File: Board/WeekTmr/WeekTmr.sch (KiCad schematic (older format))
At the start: 18 parts, among them J1 Screw_Terminal_01x03, J2 Screw_Terminal_01x03, J3 Barrel_Jack_MountingPin, J4 DS3231, K1 DIPxx-1Cxx-51x, K2 DIPxx-1Cxx-51x, Q1 BC817, Q2 BC817, SW1 DOWN_BUT, SW2 UP_BUT, SW3 SELECT_BUT, U1 NHD-0420H1Z

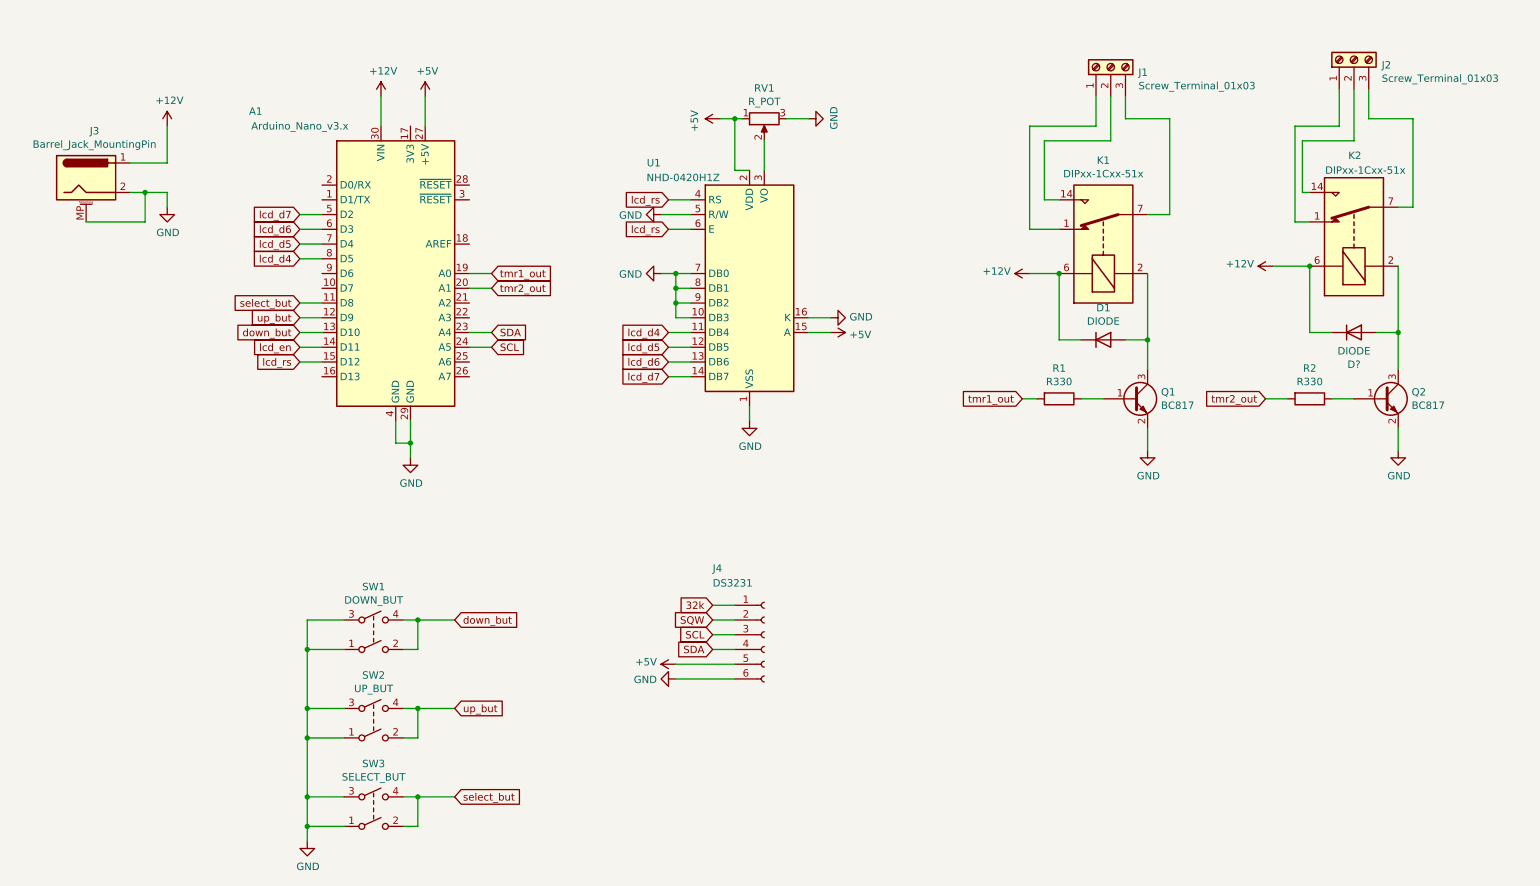
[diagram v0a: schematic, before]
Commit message: pcb update
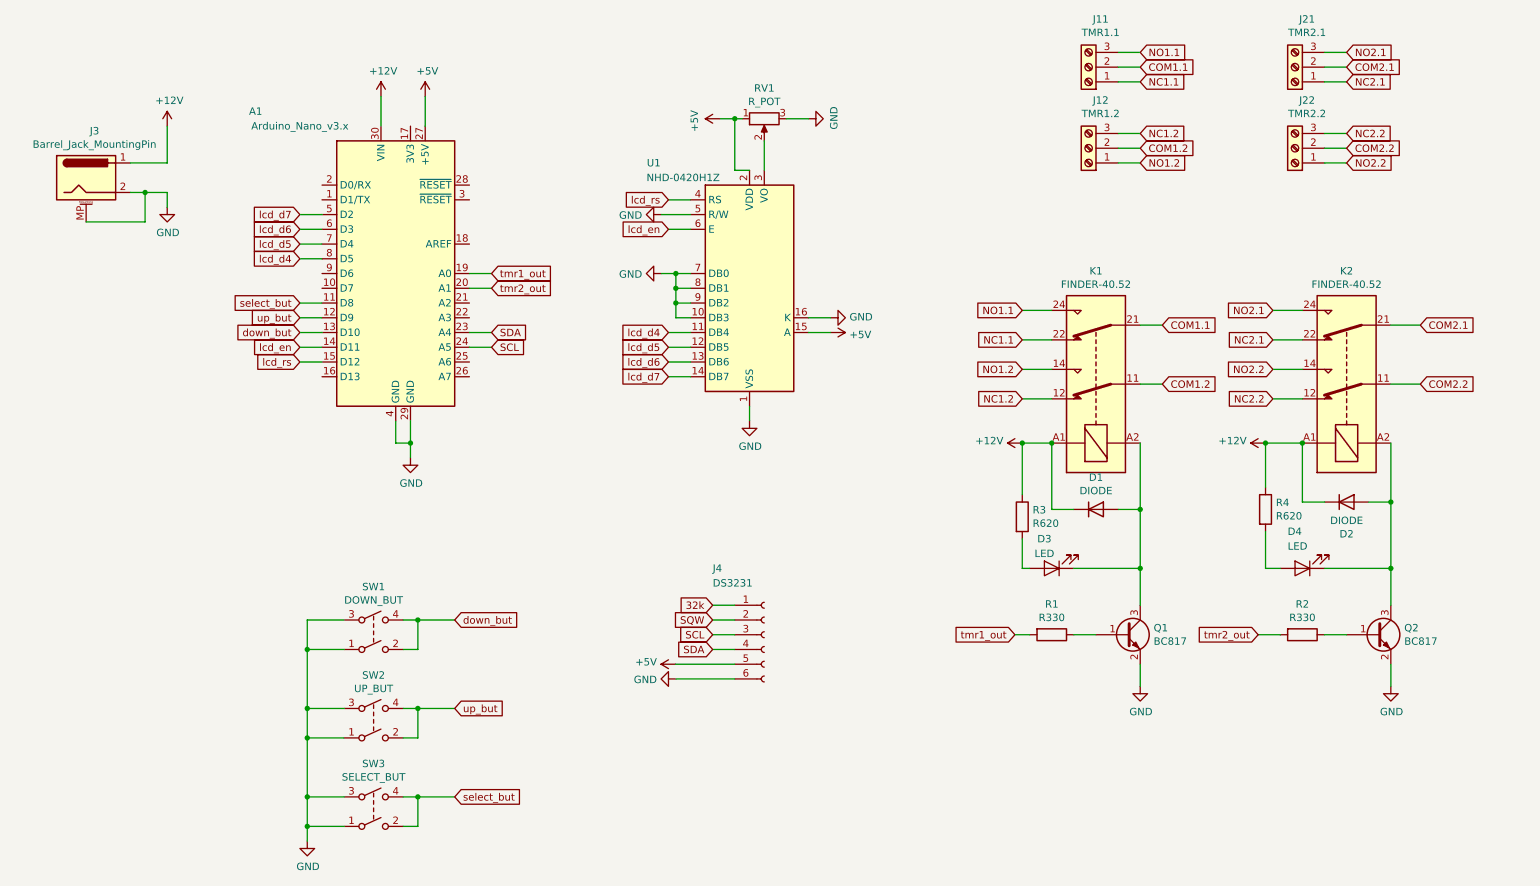
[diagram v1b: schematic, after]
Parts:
- removed J1, J2: Screw_Terminal_01x03, symbol Connector:Screw_Terminal_01x03
- removed K1, K2: DIPxx-1Cxx-51x, Relay_THT:Relay_StandexMeder_DIP_LowProfile, symbol Relay:DIPxx-1Cxx-51x
- added D3, D4: LED, LED_THT:LED_D5.0mm_Clear, symbol Device:LED
- added J11: TMR1.1, TerminalBlock_Phoenix:TerminalBlock_Phoenix_MKDS-1,5-3-5.08_1x03_P5.08mm_Horizontal, symbol Connector:Screw_Terminal_01x03
- added J12: TMR1.2, TerminalBlock_Phoenix:TerminalBlock_Phoenix_MKDS-1,5-3-5.08_1x03_P5.08mm_Horizontal, symbol Connector:Screw_Terminal_01x03
- added J21: TMR2.1, TerminalBlock_Phoenix:TerminalBlock_Phoenix_MKDS-1,5-3-5.08_1x03_P5.08mm_Horizontal, symbol Connector:Screw_Terminal_01x03
- added J22: TMR2.2, TerminalBlock_Phoenix:TerminalBlock_Phoenix_MKDS-1,5-3-5.08_1x03_P5.08mm_Horizontal, symbol Connector:Screw_Terminal_01x03
- added K1, K2: FINDER-40.52, Relay_THT:Relay_DPDT_Finder_40.52, symbol Relay:FINDER-40.52
- added R3, R4: R620, Resistor_SMD:R_0805_2012Metric_Pad1.15x1.40mm_HandSolder, symbol Device:R
- D1: footprint (none) -> Diode_THT:D_DO-15_P15.24mm_Horizontal
- D2: renamed from D?; footprint (none) -> Diode_THT:D_DO-15_P15.24mm_Horizontal
- J3: footprint (none) -> KiCad_Library:BarrelJack_Horizontal_comet
- J4: footprint (none) -> KiCad_Library:DS3231_RTC_Module
- R1, R2: footprint (none) -> Resistor_SMD:R_0805_2012Metric_Pad1.15x1.40mm_HandSolder
- RV1: footprint (none) -> KiCad_Library:Pot_custom
- SW1, SW2, SW3: footprint (none) -> KiCad_Library:SW_Button
- U1: footprint Display:NHD-0420H1Z -> KiCad_Library:LCD_4x20_Stoian
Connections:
- net +12V: now also K1.A1, K2.A1, R3.1, R4.1
- net lcd_en: now also U1.6 (E)
- net lcd_rs: no longer U1.6 (E)
- net at D1.1 (A), Q1.3 (C): now also D3.1 (K), K1.A2
- net at D2.1 (A), Q2.3 (C): now also D4.1 (K), K2.A2
- new net: D3.2 (A), R3.2
- new net: D4.2 (A), R4.2
- new net COM1.1: J11.2 (Pin_2), K1.21
- new net COM1.2: J12.2 (Pin_2), K1.11
- new net COM2.1: J21.2 (Pin_2), K2.21
- new net COM2.2: J22.2 (Pin_2), K2.11
- new net NC1.1: J11.1 (Pin_1), K1.22
- new net NC1.2: J12.3 (Pin_3), K1.12
- new net NC2.1: J21.1 (Pin_1), K2.22
- new net NC2.2: J22.3 (Pin_3), K2.12
- new net NO1.1: J11.3 (Pin_3), K1.24
- new net NO1.2: J12.1 (Pin_1), K1.14
- new net NO2.1: J21.3 (Pin_3), K2.24
- new net NO2.2: J22.1 (Pin_1), K2.14
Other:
- moved on the sheet: D1, D2, Q1, Q2, R1, R2
